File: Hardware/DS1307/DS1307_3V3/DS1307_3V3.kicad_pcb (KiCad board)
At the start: 2 copper layers, 9 parts, among them P1 I2C, U1 DS1307, X1 32.768kHz

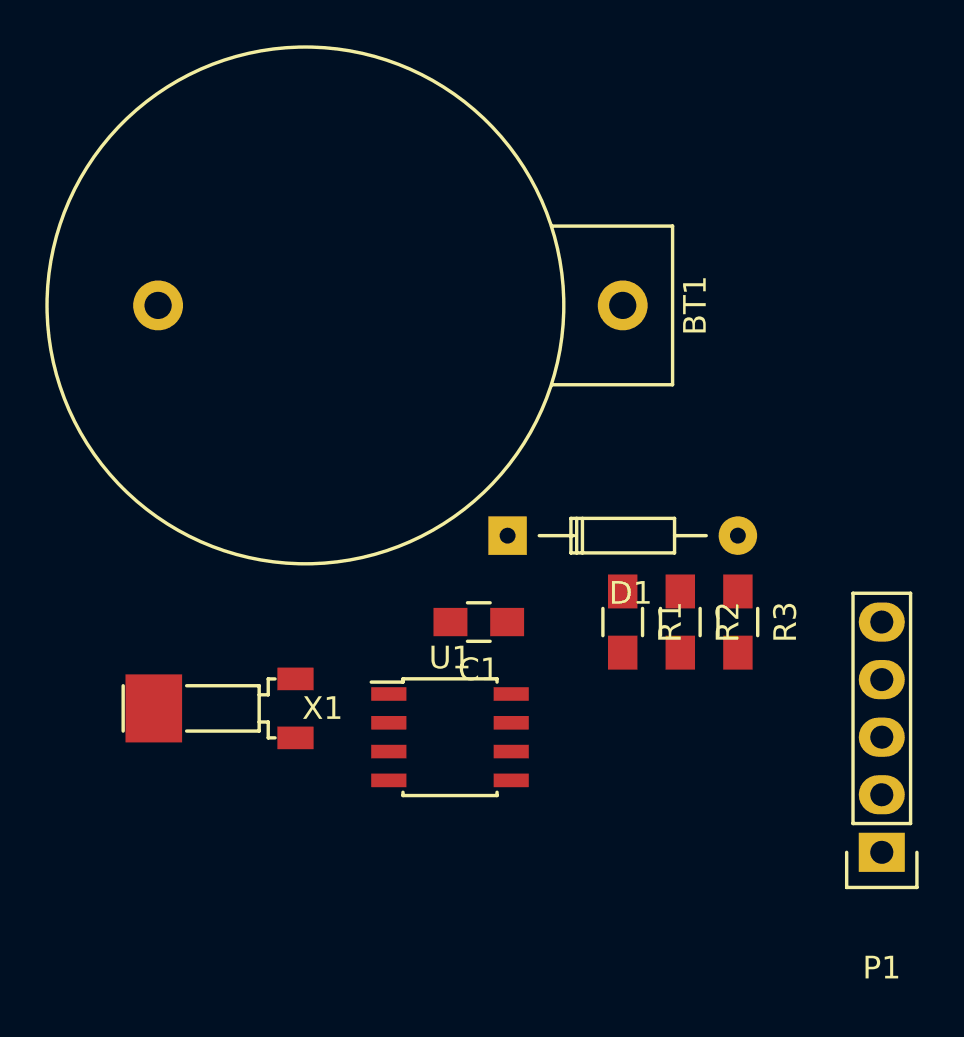
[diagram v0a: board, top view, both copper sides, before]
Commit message: work on layout
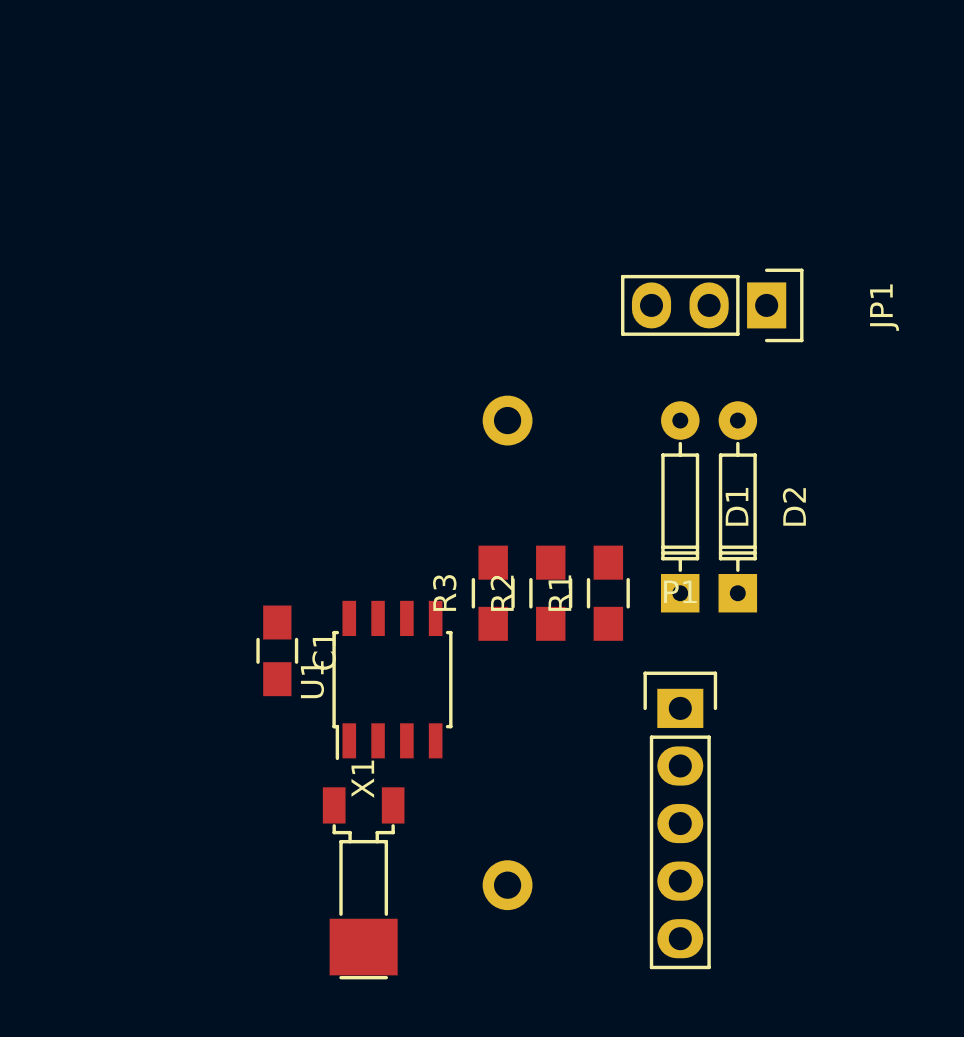
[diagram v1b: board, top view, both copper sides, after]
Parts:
- added D2: D, Diodes_ThroughHole:Diode_DO-35_SOD27_Horizontal_RM7.5, F.Cu at (127.0, 59.7)
- added JP1: Diode, Pin_Headers:Pin_Header_Straight_1x03, F.Cu at (128.3, 47.0)
- BT1: moved to B.Cu
- D1: footprint Diodes_ThroughHole:Diode_DO-35_SOD27_Horizontal_RM10 -> Diodes_ThroughHole:Diode_DO-35_SOD27_Horizontal_RM7.5
- moved P1 10.9 mm to (124.5, 64.8), turned to 0 degrees
- moved R3 10.9 mm to (116.2, 59.7), turned to 90 degrees
- moved C1 8.98 mm to (106.7, 62.2), turned to 270 degrees
- moved D1 8.03 mm to (124.5, 59.7), turned to 90 degrees
- moved BT1 7.18 mm to (116.8, 52.1), turned to 90 degrees
- moved X1 6.35 mm to (110.5, 69.8), turned to 90 degrees
- moved R2 5.85 mm to (118.7, 59.7), turned to 90 degrees
- moved U1 3.59 mm to (111.8, 63.5), turned to 90 degrees
- moved R1 1.42 mm to (121.3, 59.7), turned to 90 degrees
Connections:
- D1 pad 1: Net-(C1-Pad1) -> Net-(D1-Pad1)
